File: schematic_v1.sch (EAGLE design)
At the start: 2 parts, among them U1 MAX7219CWGT

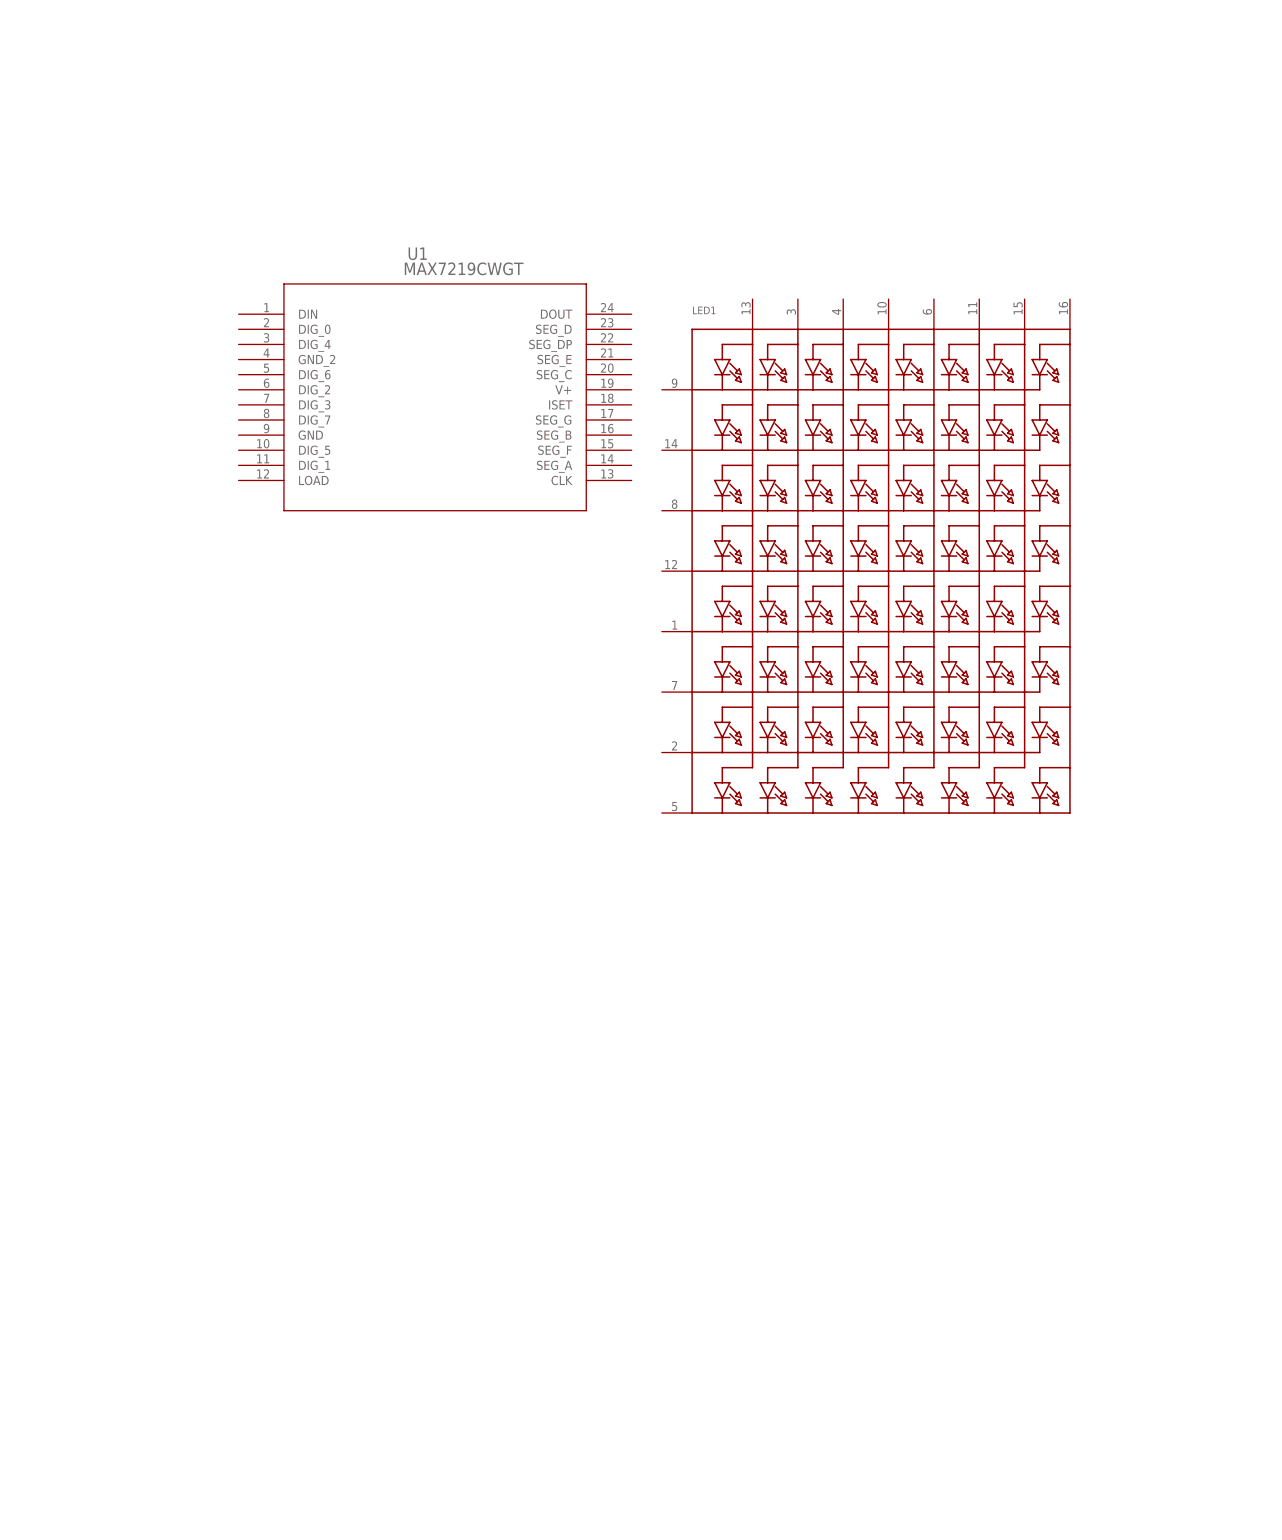
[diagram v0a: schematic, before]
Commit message: Update schematic_v1.sch
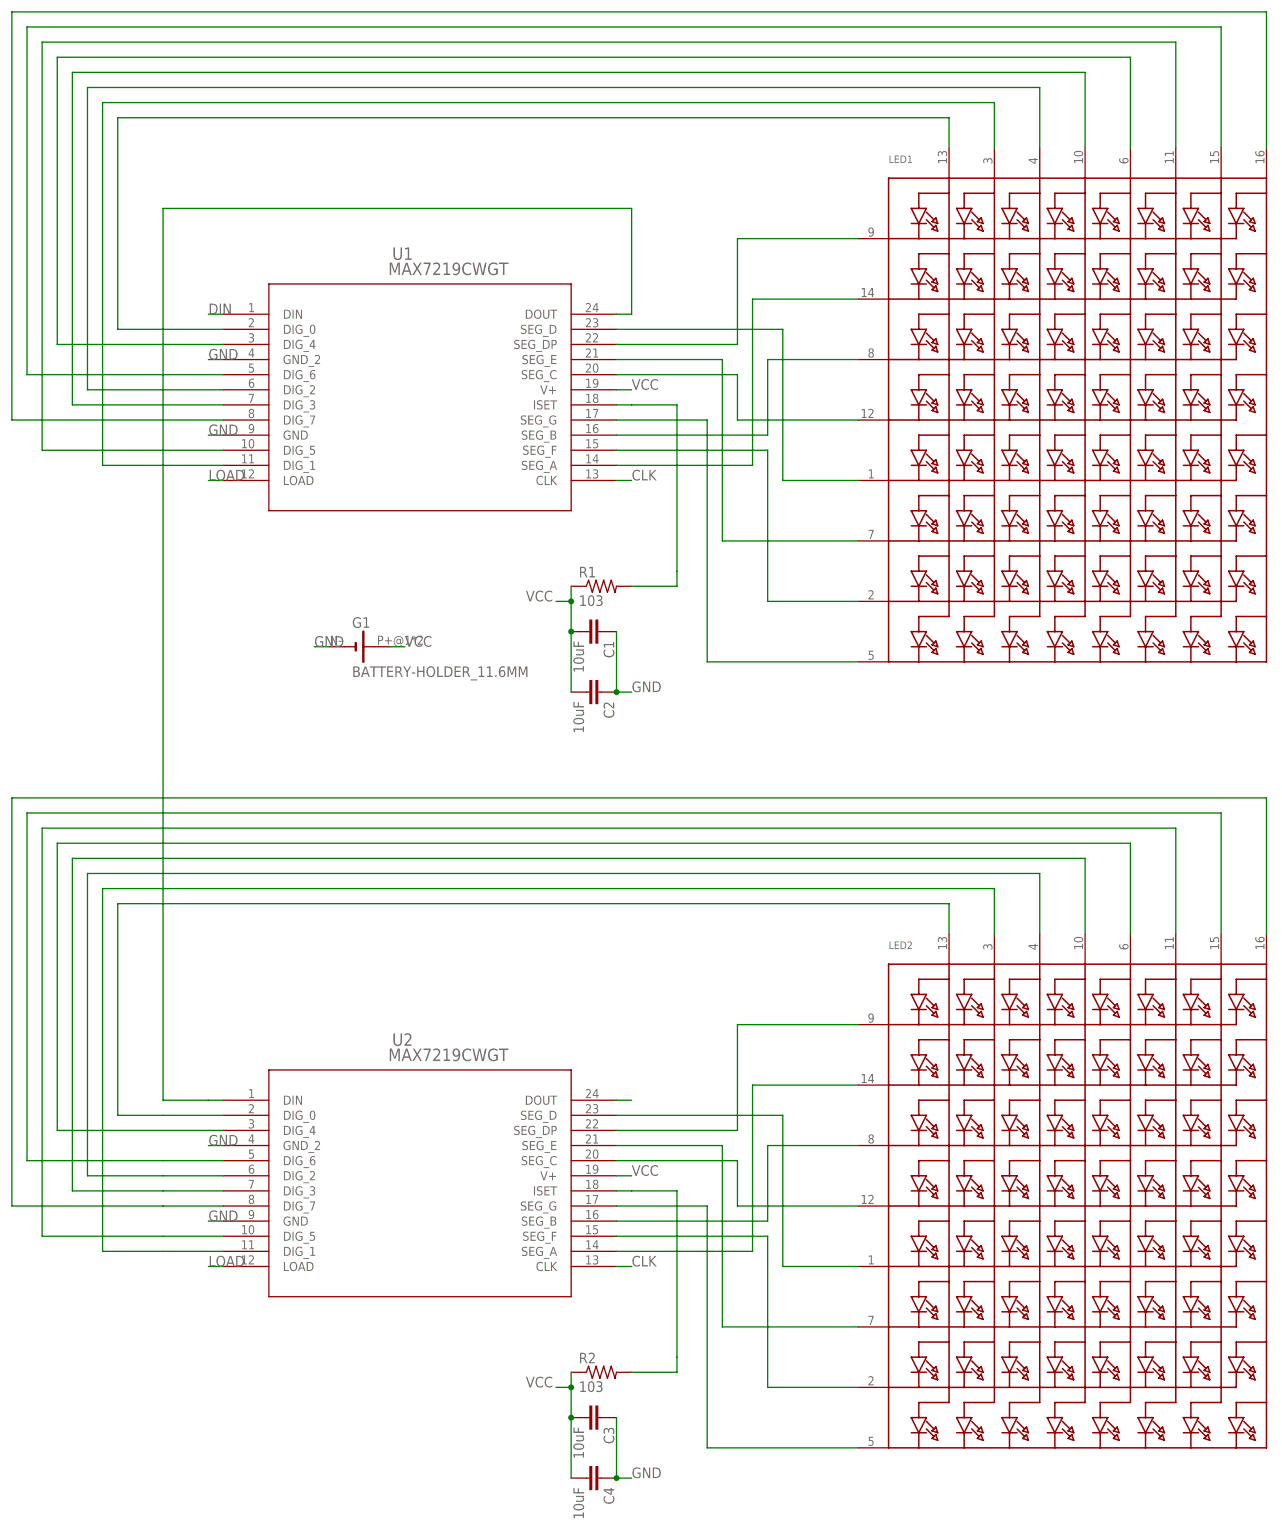
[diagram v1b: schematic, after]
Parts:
- added C1, C2, C3, C4: 10uF, SparkFun-Capacitors:10UF-0805-10V-10%
- added G1: BATTERY-HOLDER_11.6MM, battery:BATTERY-HOLDER_11.6MM
- added LED2: (no value), adafruit:SEGMENT_8X8_ROWCATHODEBL-M15
- added R1, R2: 103, adafruit:R-US_M0805
- added U2: MAX7219CWGT, MAX7219CWGT:MAX7219CWGT
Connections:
- new net CLK: U1.CLK, U2.CLK
- new net DIN: U1.DIN
- new net GND: C1.1, C2.1, C3.1, C4.1, G1.-, U1.GND, U1.GND_2, U2.GND, U2.GND_2
- new net LOAD: U1.LOAD, U2.LOAD
- new net N$10: LED1.A6, U1.DIG_5
- new net N$11: LED1.A2, U1.DIG_1
- new net N$12: LED2.A5, U2.DIG_4
- new net N$13: LED1.K1, U1.SEG_DP
- new net N$14: LED1.K2, U1.SEG_A
- new net N$15: LED1.K3, U1.SEG_B
- new net N$16: LED1.K4, U1.SEG_C
- new net N$17: LED1.K5, U1.SEG_D
- new net N$18: LED1.K6, U1.SEG_E
- new net N$19: LED1.K7, U1.SEG_F
- new net N$2: LED1.A1, U1.DIG_0
- new net N$20: LED1.K8, U1.SEG_G
- new net N$21: U1.DOUT, U2.DIN
- new net N$22: LED2.A7, U2.DIG_6
- new net N$23: R1.2, U1.ISET
- new net N$24: LED2.A3, U2.DIG_2
- new net N$25: LED2.A4, U2.DIG_3
- new net N$26: LED2.A8, U2.DIG_7
- new net N$27: LED2.A6, U2.DIG_5
- new net N$28: LED2.A2, U2.DIG_1
- new net N$29: LED2.K1, U2.SEG_DP
- new net N$3: LED1.A5, U1.DIG_4
- new net N$30: LED2.K2, U2.SEG_A
- new net N$31: LED2.K3, U2.SEG_B
- new net N$32: LED2.K4, U2.SEG_C
- new net N$33: LED2.K5, U2.SEG_D
- new net N$34: LED2.K6, U2.SEG_E
- new net N$35: LED2.K7, U2.SEG_F
- new net N$36: LED2.K8, U2.SEG_G
- new net N$37: U2.DOUT
- new net N$38: R2.2, U2.ISET
- new net N$5: LED1.A7, U1.DIG_6
- new net N$6: LED1.A3, U1.DIG_2
- new net N$7: LED1.A4, U1.DIG_3
- new net N$8: LED1.A8, U1.DIG_7
- new net N$9: LED2.A1, U2.DIG_0
- new net VCC: C1.2, C2.2, C3.2, C4.2, G1.+, R1.1, R2.1, U1.V+, U2.V+
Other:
- moved on the sheet: LED1, U1
